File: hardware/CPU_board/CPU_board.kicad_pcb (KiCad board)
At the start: 4 copper layers, 51.5 x 25.8 mm, 101 parts, among them J1 TF 1.5H 短体, J2 DF12NB_3.0_-30DS-0.5V_51, J3 DF12NB_3.0_-30DS-0.5V_51, J4 JTAG, J5 Conn_01x03, J6 Conn_01x6_Male, J7 Conn_01x03, U1 EA3036A, U2 W25Q32JVZPIQ, U3 D1s-eLQFP128, U5 PAD30, U6 PAD30, U7 PAD30, X1 24MHz, X2 32.768KHz

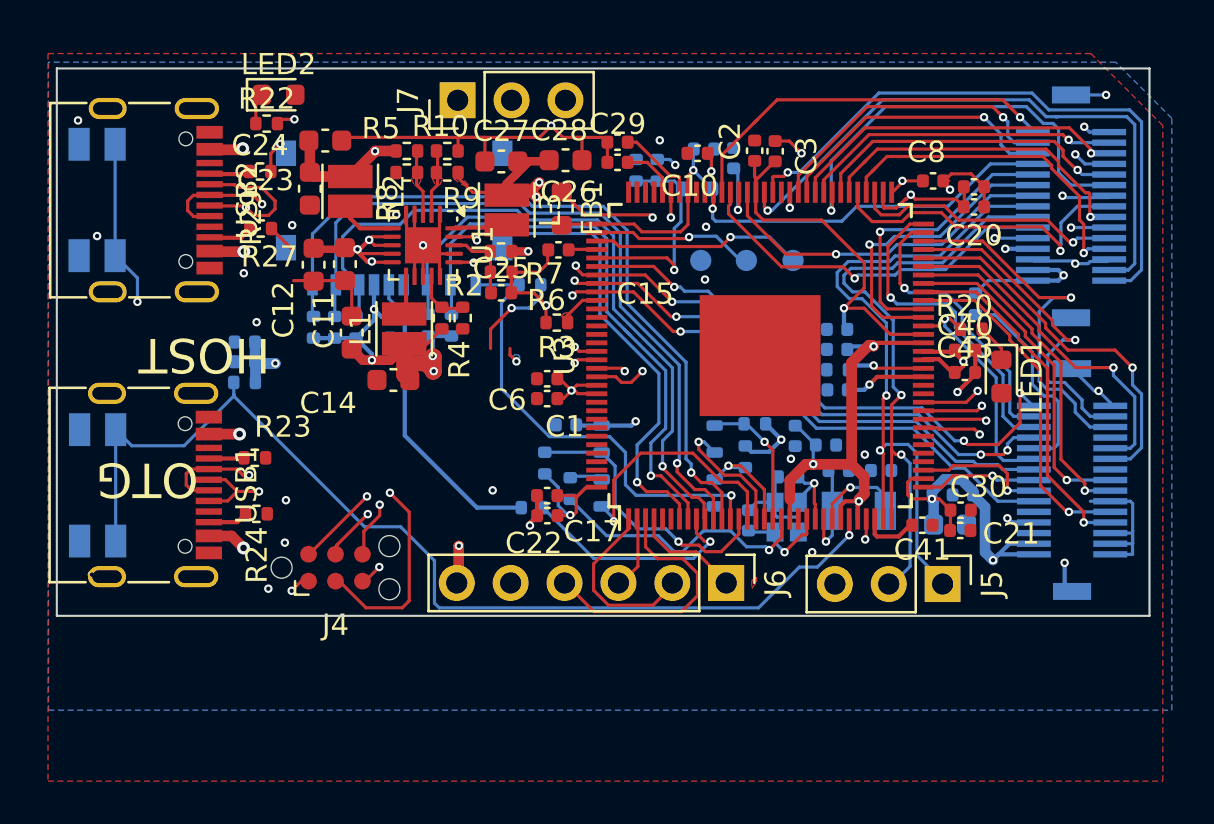
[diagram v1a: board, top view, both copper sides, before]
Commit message: update PCB design files
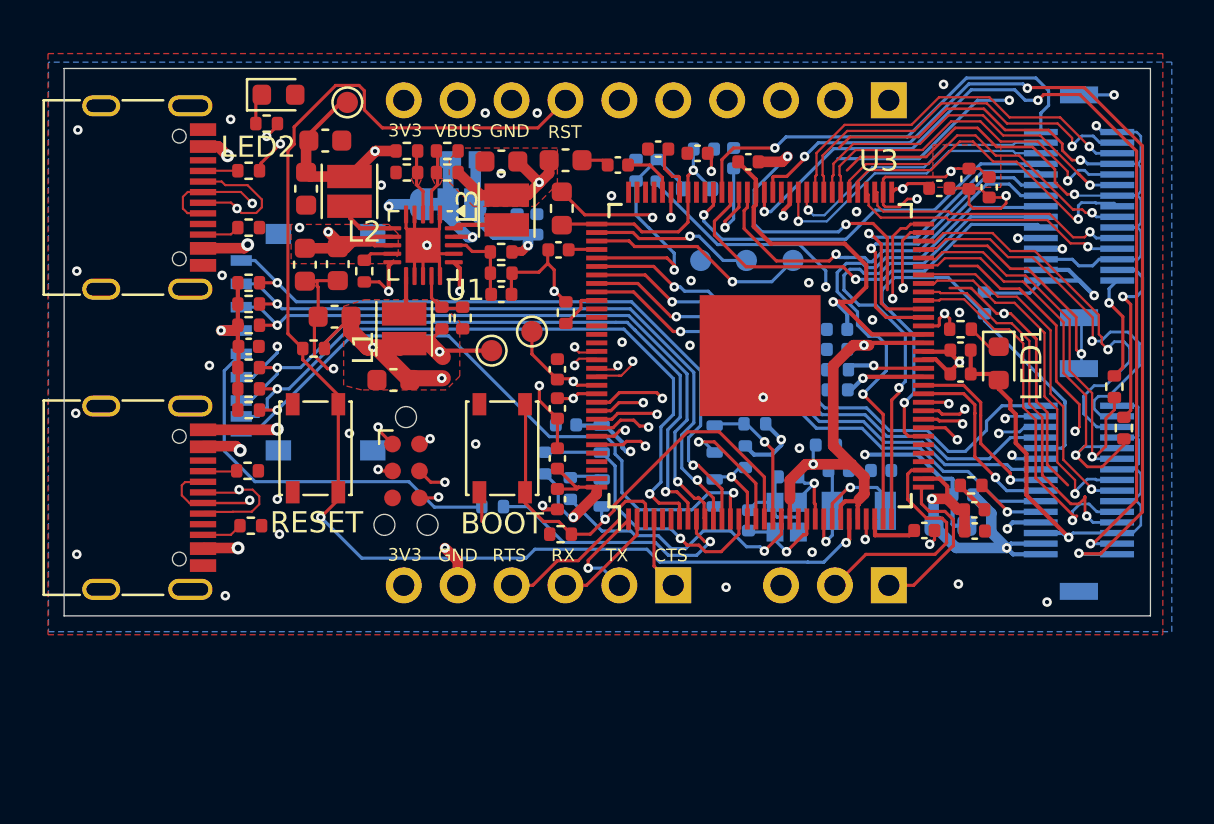
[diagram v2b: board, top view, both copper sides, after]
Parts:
- removed C42: 10u, Capacitor_SMD:C_0603_1608Metric
- removed C44: 0.1uF, Capacitor_SMD:C_0402_1005Metric
- removed J7: Conn_01x03, Connector_PinHeader_2.54mm:PinHeader_1x03_P2.54mm_Vertical
- added D2: D_Schottky, Library:U-DFN1608-2_L1.6-W0.8-RD, B.Cu at (82.3, 95.0)
- added G***: LOGO, LOGO, B.Cu at (102.7, 101.8)
- added G***: LOGO, LOGO, B.Cu at (73.8, 112.9)
- added J8: Conn_01x10_Male, Connector_PinHeader_2.54mm:PinHeader_1x10_P2.54mm_Vertical, B.Cu at (102.4, 92.2)
- added JP1: SolderJumper_3_Bridged12, Jumper:SolderJumper-3_P1.3mm_Bridged12_RoundedPad1.0x1.5mm, B.Cu at (81.6, 97.1)
- added R18: 100k, Resistor_SMD:R_0402_1005Metric, F.Cu at (77.7, 100.3)
- added R30: 10K, Library:R_0402_1005Metric, B.Cu at (106.9, 101.8)
- added R31: 10k, Resistor_SMD:R_0402_1005Metric, F.Cu at (86.9, 112.7)
- added R33: 22, Resistor_SMD:R_0402_1005Metric, F.Cu at (113.0, 105.7)
- added R34: 22, Resistor_SMD:R_0402_1005Metric, F.Cu at (113.5, 107.7)
- added U4: PAD30, TestPoint:TestPoint_Pad_D1.0mm, F.Cu at (83.7, 104.0)
- added U8: PAD30, TestPoint:TestPoint_Pad_D1.0mm, F.Cu at (76.9, 92.3)
- added U9: PAD30, TestPoint:TestPoint_Pad_D1.0mm, F.Cu at (85.6, 103.1)
- C2: value 0.1uF -> 10u; footprint Capacitor_SMD:C_0402_1005Metric -> Capacitor_SMD:C_0603_1608Metric; moved to B.Cu
- C31, R1, R11, R13, R14, R15, R17, R19: moved to F.Cu
- FEL1: value EVQPUJ_EVQPUA -> FEL; footprint Button_Switch_SMD:Panasonic_EVQPUJ_EVQPUA -> Button_Switch_SMD:SW_SPST_PTS810; moved to F.Cu
- J1: value TF 1.5H 短体 -> TF TF-018 1.5mm; footprint Project_YuzukiNezha D1s - RISC-V Linux 核心板_2022-01-07_23-15-16:TFCARD 短体 1.5H -> Library:TF-SMD_TF-018
- J2: value DF12NB_3.0_-30DS-0.5V_51 -> SOUTH
- J3: value DF12NB_3.0_-30DS-0.5V_51 -> NORTH
- J4: value JTAG -> Conn_01x6_Male; footprint Connector:Tag-Connect_TC2030-IDC-NL_2x03_P1.27mm_Vertical -> Connector_PinHeader_2.54mm:PinHeader_1x06_P2.54mm_Vertical; moved to B.Cu
- J5: moved to B.Cu
- J6: value Conn_01x6_Male -> JTAG; footprint Connector_PinHeader_2.54mm:PinHeader_1x06_P2.54mm_Vertical -> Connector:Tag-Connect_TC2030-IDC-NL_2x03_P1.27mm_Vertical
- LED2: value LED-0603_ORANGE -> LED-0603_PURPLE
- R22: value 5k1 -> 3k3
- R26: value 10K -> 84.5K 1%; moved to F.Cu
- RESET1: value EVQPUJ_EVQPUA -> RESET; footprint Button_Switch_SMD:Panasonic_EVQPUJ_EVQPUA -> Button_Switch_SMD:SW_SPST_PTS810; moved to F.Cu
- U1: footprint Package_DFN_QFN:WQFN-20-1EP_3x3mm_P0.4mm_EP1.7x1.7mm -> Package_DFN_QFN:QFN-20-1EP_3x3mm_P0.4mm_EP1.65x1.65mm
- moved FEL1 22.4 mm to (84.2, 108.6), turned to 90 degrees
- moved C2 19.9 mm to (105.3, 112.3), turned to 180 degrees
- moved J6 16.0 mm to (79.7, 109.7)
- moved J4 15.9 mm to (92.3, 115.1), turned to 90 degrees
- moved C39 14.8 mm to (85.8, 98.1), turned to -90 degrees
- moved R15 14.5 mm to (72.2, 106.8), turned to 0 degrees
- moved C38 14.4 mm to (84.9, 98.1), turned to -90 degrees
- moved USB2 14.0 mm to (66.4, 110.9)
- moved USB1 13.6 mm to (66.4, 96.8)
- moved RESET1 10.4 mm to (75.4, 108.6), turned to 90 degrees
- moved R1 10.0 mm to (72.2, 105.8), turned to 0 degrees
- moved R11 8.69 mm to (72.2, 104.8), turned to 0 degrees
- moved R26 8.55 mm to (106.3, 110.4), turned to 0 degrees
- moved J1 8.06 mm to (75.0, 103.6), turned to 90 degrees
- moved C31 6.72 mm to (72.2, 103.8), turned to 180 degrees
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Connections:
- net /D0+ renamed /USB_D0+
- net /D0- renamed /USB_D0-
- net /D1+ renamed /USB_D1+
- net /D1- renamed /USB_D1-
- net /LCD_D10 renamed /LCD_CKP
- net /LCD_D11 renamed /LCD_CKN
- net /LCD_D12 renamed /LCD_V3P
- net /LCD_D13 renamed /LCD_V3N
- net /LCD_D14 renamed /LCD_U0P
- net /LCD_D15 renamed /LCD_U0N
- net /LCD_D18 renamed /LCD_U1P
- net /LCD_D19 renamed /LCD_U1N
- net /LCD_D2 renamed /LCD_V0P
- net /LCD_D20 renamed /LCD_U2P
- net /LCD_D21 renamed /LCD_U2N
- net /LCD_D22 renamed /LCD_UCKP
- net /LCD_D23 renamed /LCD_UCKN
- net /LCD_D3 renamed /LCD_V0N
- net /LCD_D4 renamed /LCD_V1P
- net /LCD_D5 renamed /LCD_V1N
- net /LCD_D6 renamed /LCD_V2P
- net /LCD_D7 renamed /LCD_V2N
- net /SPI0_D1 renamed /SDC2_D1
- net /SPI0_D3 renamed /SDC2_D3
- net Net-(U3-LDOB-OUT) renamed /LDO_BOUT
- C11 pad 2: VBUS -> VSYS
- C12 pad 2: VBUS -> VSYS
- C2 pad 1: 0V9 -> GND
- C2 pad 2: GND -> 3V3
- FEL1 pad 2: /SPI0_D2 -> /SDC2_D2
- J2 pad 28: GND -> /LCD_D16
- J2 pad 30: GND -> /LCD_D17
- J2 pad 9: Net-(J2-Pad9) -> /PSEL
- J3 pad 28: /LCD_D16 -> /B6
- J3 pad 3: /LCD_DE -> /LCD_U3P
- J3 pad 30: /LCD_D17 -> /B7
- J3 pad 5: /LCD_CLK -> /LCD_U3N
- J4 pad 1: 3V3 -> /CTS1
- J4 pad 2: /JTAG_TMS -> /TX1
- J4 pad 3: /JTAG_TDI -> /RX1
- J4 pad 4: /JTAG_TCK -> /RTS1
- J4 pad 6: /JTAG_TDO -> 3V3
- J5 pad 1: /SDA -> /RX0
- J5 pad 2: /SCK -> /TX0
- J6 pad 1: /CTS1 -> 3V3
- J6 pad 2: /TX1 -> /JTAG_TMS
- J6 pad 3: /RX1 -> /JTAG_TDI
- J6 pad 4: /RTS1 -> /JTAG_TCK
- J6 pad 6: 3V3 -> /JTAG_TDO
- R1 pad 1: /SDC0_D1 -> 3V3
- R1 pad 2: 3V3 -> /SDC0_D1
- R11 pad 1: /SDC0_D0 -> 3V3
- R11 pad 2: 3V3 -> /SDC0_D0
- R13 pad 1: /SDC0_D3 -> 3V3
- R13 pad 2: 3V3 -> /SDC0_D3
- R17 pad 1: /SDC0_D2 -> 3V3
- R17 pad 2: 3V3 -> /SDC0_D2
- R23 pad 2: Net-(USB1-CC1) -> Net-(USB2-CC1)
- R24 pad 1: Net-(USB1-CC2) -> Net-(USB2-CC2)
- R26 pad 1: Net-(J2-Pad9) -> GND
- R26 pad 2: 3V3 -> Net-(J2-Pad21)
- R27 pad 1: GND -> Net-(USB1-CC2)
- R27 pad 2: Net-(USB2-CC2) -> GND
- R29 pad 1: Net-(USB2-CC1) -> GND
- R29 pad 2: GND -> Net-(USB1-CC1)
- R37 pad 2: /SPI0_D2 -> /SDC2_D0
- U1 pad 16: VBUS -> VSYS
- U1 pad 19: VBUS -> VSYS
- U1 pad 7: VBUS -> VSYS
- U1 pad 8: VBUS -> VSYS
- U1 pad 9: VBUS -> Net-(U1-EN1)
- U2 pad 3: /SPI0_D2 -> /SDC2_D0
- U2 pad 5: /SPI0_D0 -> /SDC2_D2
- U3 pad 118: unconnected-(U3-PG1-Pad118) -> /PG1
- U3 pad 119: unconnected-(U3-PG2-Pad119) -> /PG2
- U3 pad 120: unconnected-(U3-PG0-Pad120) -> /PG0
- U3 pad 121: unconnected-(U3-PG3-Pad121) -> /PG3
- U3 pad 122: unconnected-(U3-PG5-Pad122) -> /PG5
- U3 pad 123: unconnected-(U3-PG4-Pad123) -> /PG4
- U3 pad 15: /SPI0_D0 -> /SDC2_D0
- U3 pad 17: /SPI0_D2 -> /SDC2_D2
- U3 pad 33: /SDA2 -> /RX0
- U3 pad 35: /SCK2 -> /TX0
- U3 pad 39: /PE8 -> /PSEL
- U3 pad 44: /PE0 -> /SCK2
- U3 pad 45: /PE1 -> /SDA2
- U3 pad 75: /LCD_CLK -> /LCD_U3P
- U3 pad 76: /LCD_DE -> /LCD_U3N
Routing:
- net 3V3: track 79.9 -> 213.4 mm, vias 20 -> 19
- net GND: track 85.0 -> 210.5 mm, vias 34 -> 55
- net /SPI0_D2: track 50.8 -> 0.00 mm, vias 2 -> 0
- net /PG4: track 0.00 -> 25.1 mm, vias 0 -> 1
- net /PG5: track 0.00 -> 24.0 mm, vias 0 -> 1
- net VSYS: track 0.00 -> 24.0 mm, vias 0 -> 3
- net /PG0: track 0.00 -> 23.4 mm, vias 0 -> 1
- net /PSEL: track 0.00 -> 23.2 mm, vias 0 -> 1
- net /PG3: track 0.00 -> 23.2 mm, vias 0 -> 1
- net /SDC2_D2: track 0.00 -> 22.3 mm, vias 0 -> 1
- net /PG2: track 0.00 -> 22.1 mm, vias 0 -> 1
- net /PG1: track 0.00 -> 21.9 mm, vias 0 -> 1
- net /LCD_D17: track 28.9 -> 44.1 mm, vias 1 -> 3
- net VBUS: track 121.5 -> 106.8 mm, vias 11 -> 8
- net /LCD_DE: track 14.3 -> 0.00 mm, vias 1 -> 0
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- added copper zone on In2.Cu, net 0V9
- added copper zone on In1.Cu, net 1V8
- added copper zone on In1.Cu, net 1V8_DRAM
- added copper zone on F.Cu, net 3V3
- added copper zone on In2.Cu, net 3V3
- added copper zone on In1.Cu, net VBUS
- added copper zone on F.Cu, net VSYS
- added copper zone on In1.Cu, net VSYS
- removed copper zone on B.Cu, net (none)
- removed copper zone on F.Cu, net /DXOUT
- removed copper zone on F.Cu, net Net-(U3-NC0)
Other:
- board size 51.5 x 25.8 mm -> 51.2 x 25.8 mm
- board text added: "3.3V"
- board text added: "3V3"
- board text added: "BOOT"
- board text added: "CPU board"
- board text added: "CTS"
- board text added: "GND"
- board text added: "Memory Card"
- board text added: "NOTE: currently 3313 for 6 layer LVDS impedance JLC04161H-3313 (1.56mm) 100ohm differential coplanar L1: width 0.1092mm separation 0.1778mm clearance 0.1270mm 90ohm differential non-coplanar L3: 0.1016 width (4 mil), 0.1029mm separation (4.05mil) =================== JLC04161H-1080(Finished thickness 1.52mm) 100 ohm coplanar differential L1: width .1016mm (4 mil), spacing .3581mm, clearance .1016m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"
- board text added: "RESET"
- board text added: "RST"
- board text added: "RTS"
- board text added: "RX"
- board text added: "TX"
- board text added: "VBUS"
